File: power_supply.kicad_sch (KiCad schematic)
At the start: 38 parts, among them U1 2.2uH, U3 TPS62151, U4 2.2uH, U5 TPS62151

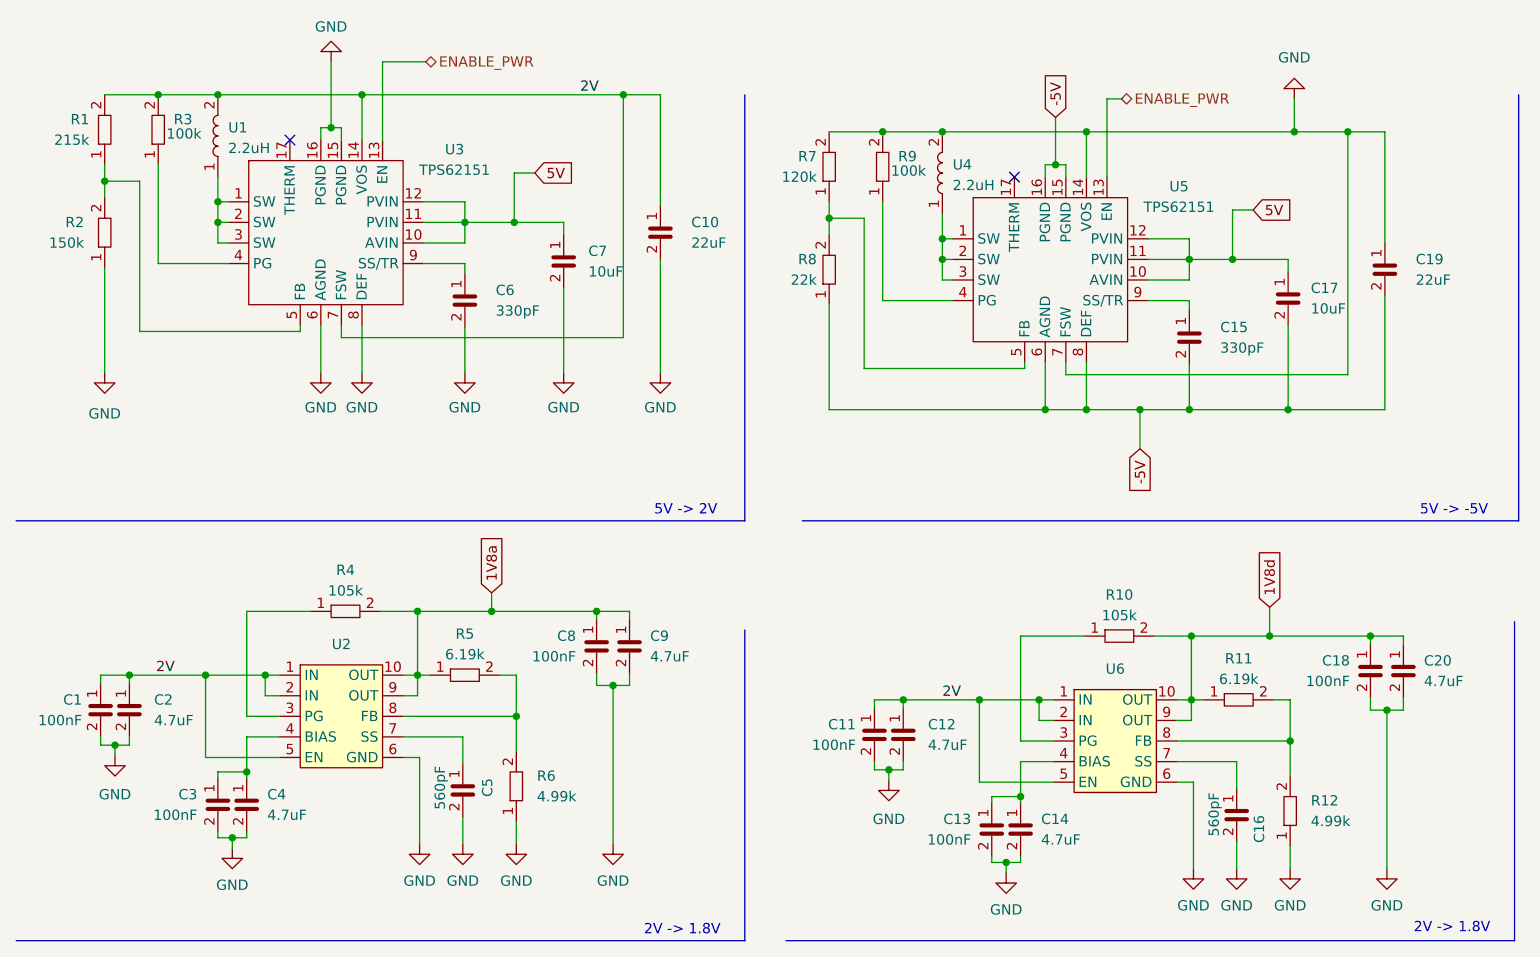
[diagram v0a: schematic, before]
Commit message: Schematic finished, ready for review.
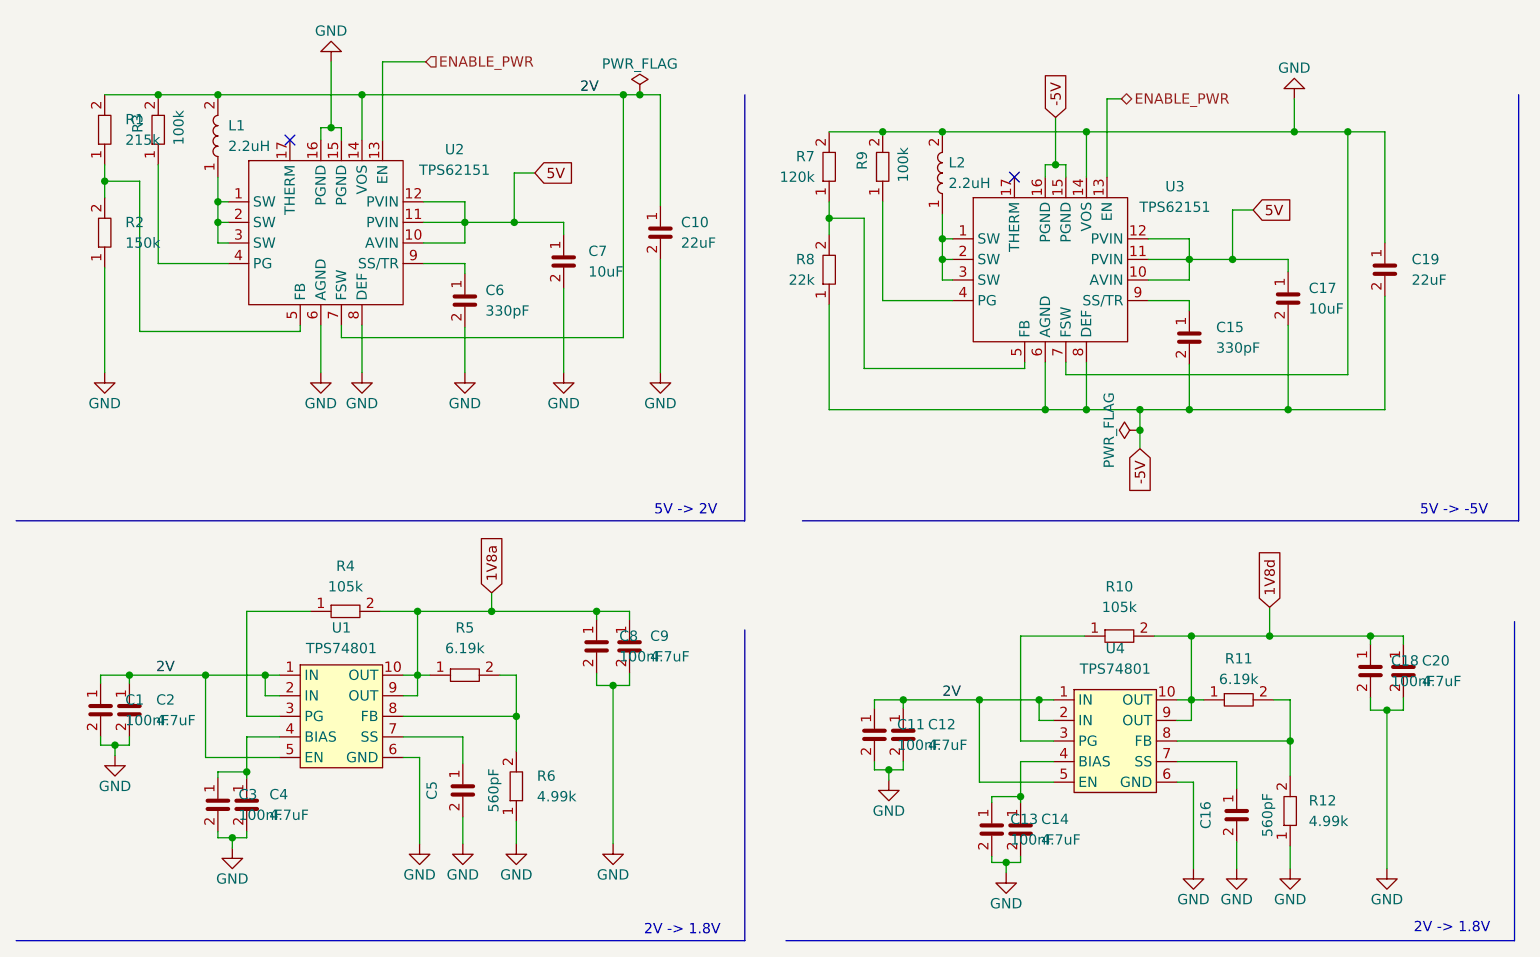
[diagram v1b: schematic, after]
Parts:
- U1: renamed from U2; value ~ -> TPS74801
- U4: renamed from U6; value ~ -> TPS74801
- renumbered U1 to L1, U4 to L2, U3 to U2, U5 to U3
